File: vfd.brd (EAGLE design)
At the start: 59 parts, among them J1 KEYPAD, J3 ARDUINO_R3, T1 8550, U1 20070-1A04PTH, X1 DRV

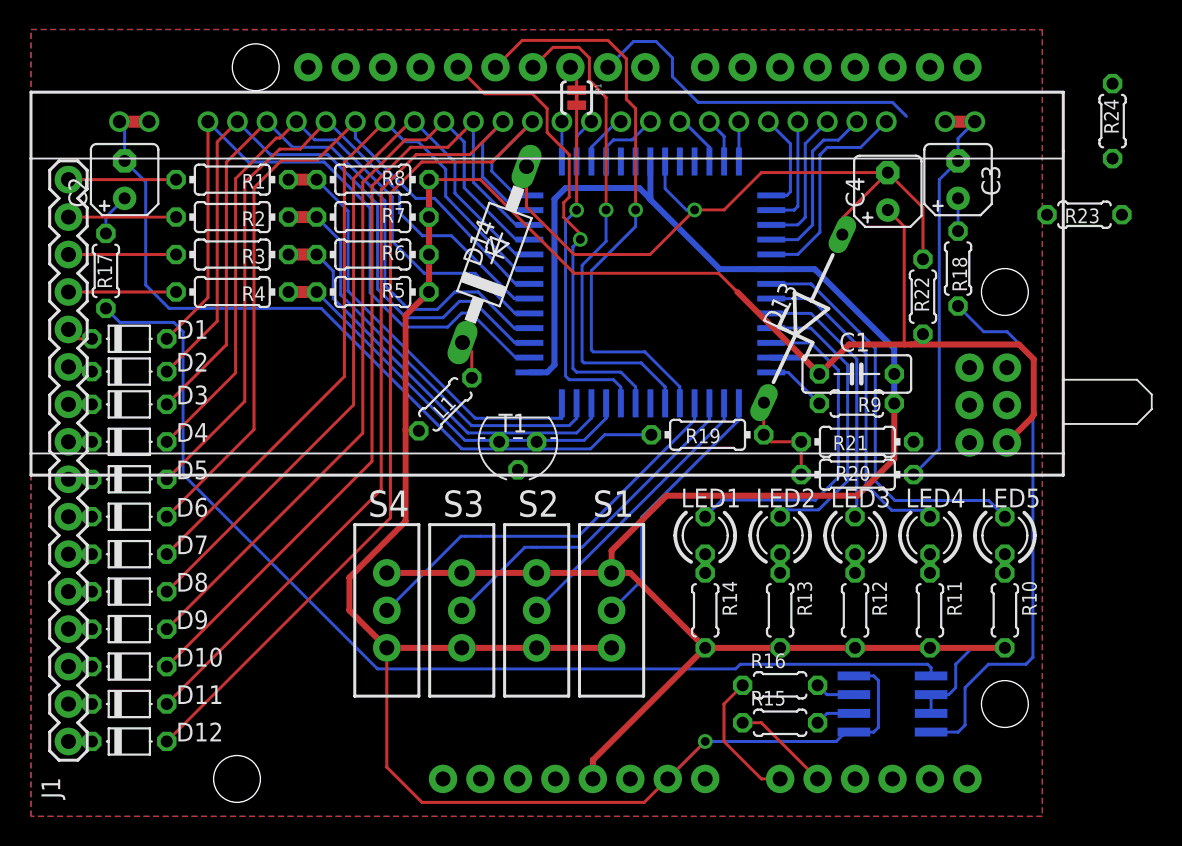
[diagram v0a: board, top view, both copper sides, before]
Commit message: all lines laid
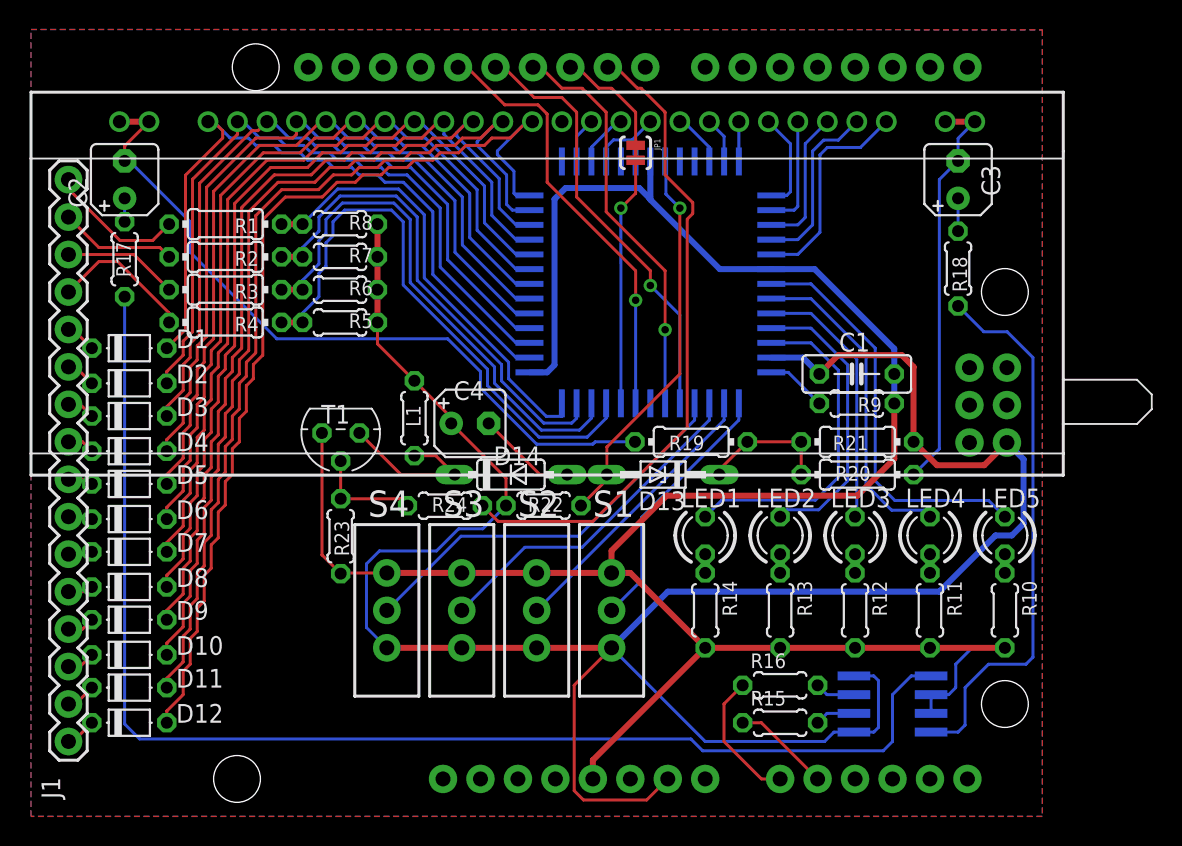
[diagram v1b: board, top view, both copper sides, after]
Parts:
- D13: device diode:ZDIO12.5 -> diode:DO34Z7
- D14: device diode:F126Z12 -> diode:DO35-7
- R5, R6, R7, R8: device resistor:0204/7 -> resistor:0204/5
- moved R23 54.9 mm to (21.0, 19.0), turned to 270 degrees
- moved R24 52.2 mm to (28.1, 21.1), turned to 0 degrees
- moved C4 32.4 mm to (29.8, 26.6), turned to 0 degrees
- moved R22 29.4 mm to (34.8, 21.1), turned to 0 degrees
- moved D14 15.0 mm to (32.5, 23.2), turned to 0 degrees
- moved D13 14.3 mm to (42.9, 23.2), turned to 180 degrees
- moved T1 12.0 mm to (21.0, 26.0)
- moved JP1 5.47 mm to (41.0, 45.0)
- moved R8 3.75 mm to (21.0, 40.2)
- moved R7 3.50 mm to (21.0, 37.9)
- moved R6 3.26 mm to (21.0, 35.7)
- moved R1 3.05 mm to (13.2, 40.2)
- moved R5 3.03 mm to (21.0, 33.5)
- moved R2 2.74 mm to (13.2, 37.9)
- moved R3 2.43 mm to (13.2, 35.7)
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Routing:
- net HVDRV: track 23.8 -> 44.4 mm
- net N$28: track 72.5 -> 88.4 mm
- net VCC: track 138.7 -> 151.9 mm
- net GND: track 172.8 -> 160.4 mm, vias 1 -> 0
- net K1: track 27.3 -> 39.0 mm
- net VEE: track 47.7 -> 36.0 mm
- net MISO: track 39.6 -> 29.4 mm
- net N$40: track 2.66 -> 10.9 mm
- net K2: track 28.1 -> 36.2 mm
- net N$36: track 0.00 -> 7.28 mm
- net SS: track 23.8 -> 16.9 mm
- net MOSI: track 33.8 -> 27.6 mm
- net N$18: track 1.73 -> 7.93 mm
- net K3: track 28.7 -> 33.3 mm
- net SEGE: track 56.1 -> 60.4 mm
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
